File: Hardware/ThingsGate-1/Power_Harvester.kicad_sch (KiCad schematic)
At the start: 3 parts, among them U14 TL082, U5 BQ24650

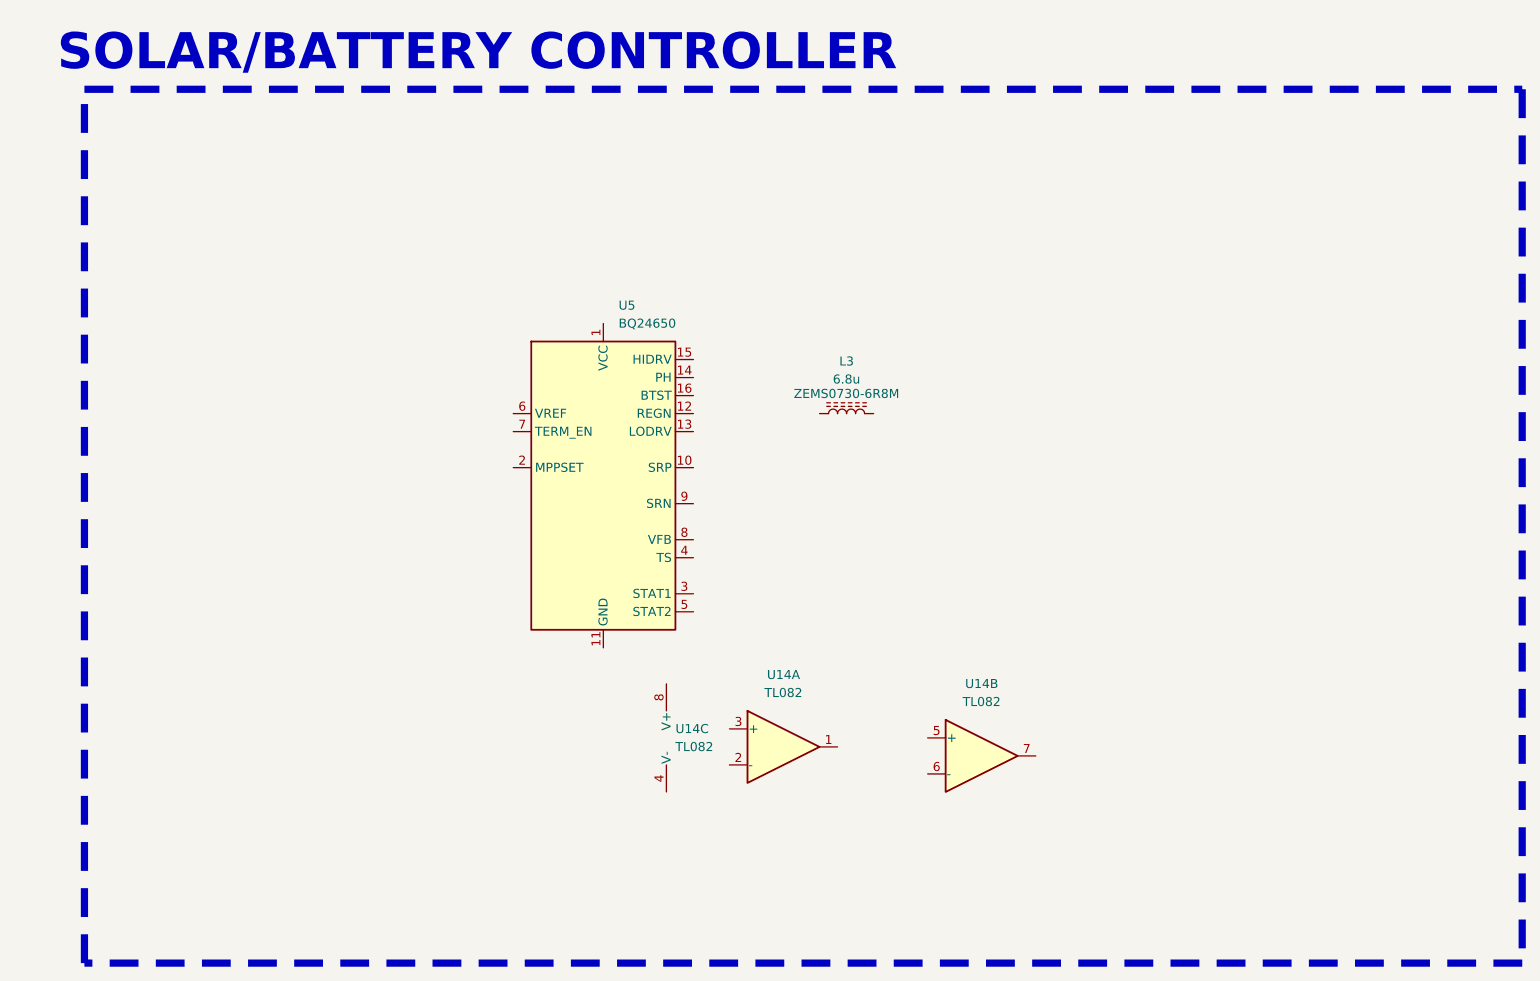
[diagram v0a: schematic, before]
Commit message: harvester schematic ready
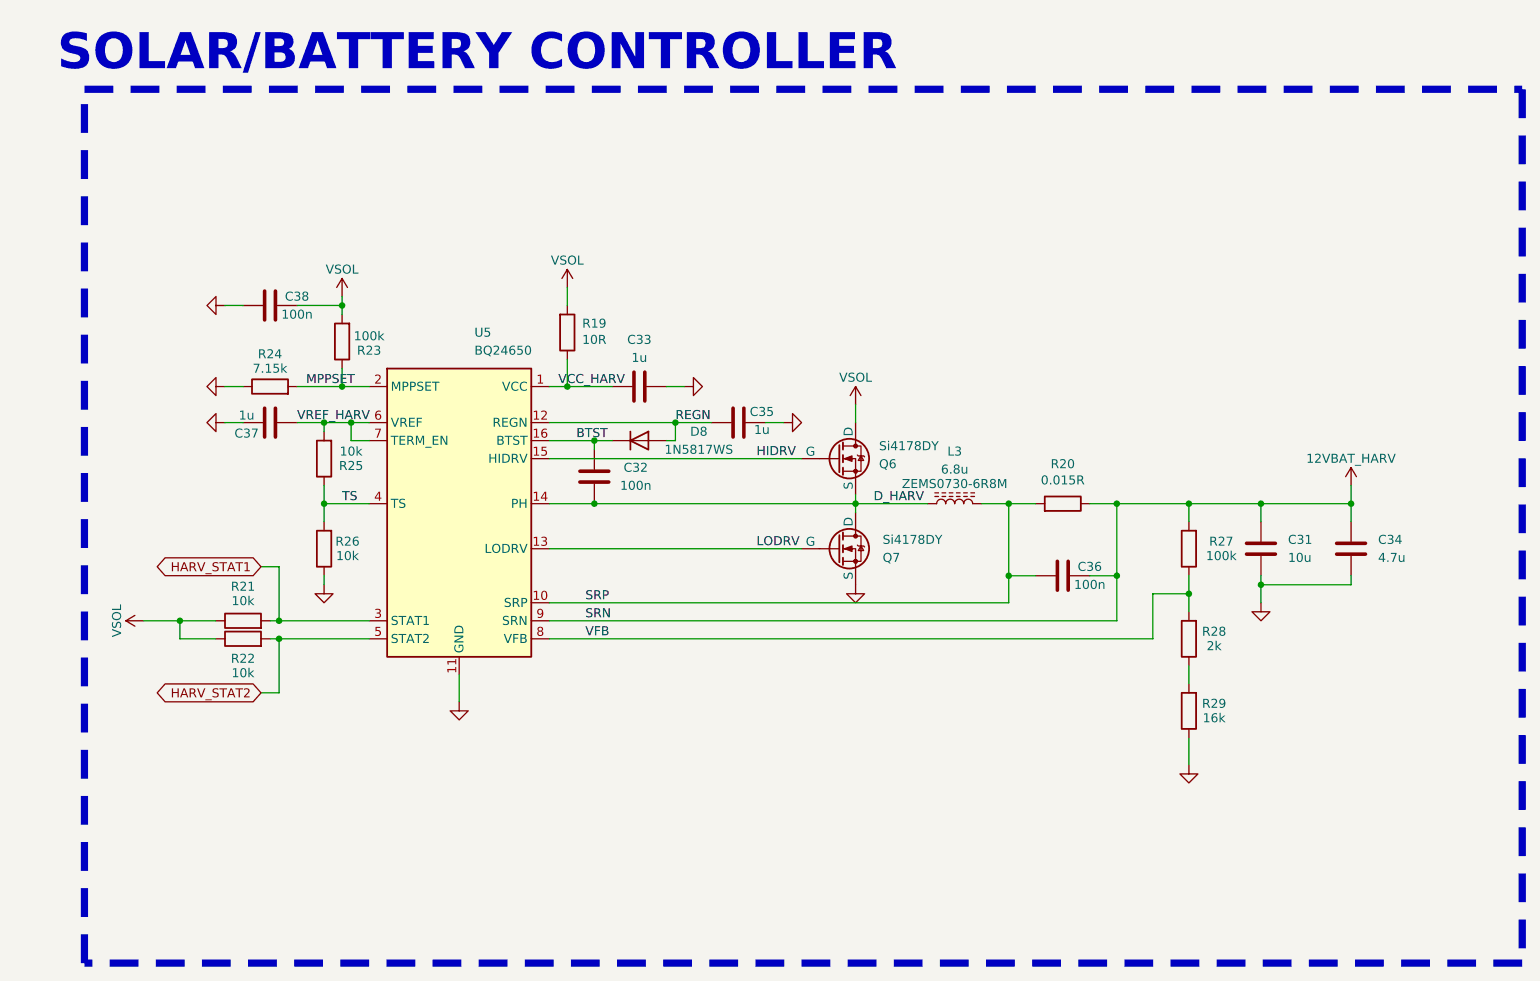
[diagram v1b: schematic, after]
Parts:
- removed U14: TL082, Package_SO:SOIC-8_3.9x4.9mm_P1.27mm, symbol Amplifier_Operational:TL082
- added C31: 10u, Fuse:Fuse_0805_2012Metric, symbol Device:C
- added C32, C36, C38: 100n, Capacitor_SMD:C_0603_1608Metric, symbol Device:C
- added C33, C35, C37: 1u, Fuse:Fuse_0805_2012Metric, symbol Device:C
- added C34: 4.7u, Fuse:Fuse_0805_2012Metric, symbol Device:C
- added D8: 1N5817WS, Diode_SMD:D_SOD-323, symbol Diode:1N4148WS
- added Q6, Q7: Si4178DY, ThingsGate-1:SO-8_3.9x4.9mm_P1.27mm, symbol ThingsGate-1:Si4178DY
- added R19: 10R, Resistor_SMD:R_1206_3216Metric, symbol Device:R
- added R20: 0.015R, Resistor_SMD:R_1206_3216Metric, symbol Device:R
- added R21, R22, R25, R26: 10k, Resistor_SMD:R_0603_1608Metric, symbol Device:R
- added R23, R27: 100k, Resistor_SMD:R_0603_1608Metric, symbol Device:R
- added R24: 7.15k, Resistor_SMD:R_0603_1608Metric, symbol Device:R
- added R28: 2k, Resistor_SMD:R_0603_1608Metric, symbol Device:R
- added R29: 16k, Resistor_SMD:R_0603_1608Metric, symbol Device:R
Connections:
- net D_HARV: now reaches L3.1
- net D_HARV: now also U5.14 (PH), C32.2, Q6.1 (S), Q6.2 (S), Q6.3 (S), Q7.5 (D), Q7.6 (D), Q7.7 (D), Q7.8 (D)
- net SRP: now reaches L3.2
- net SRP: now also U5.10 (SRP), C36.1, R20.2
- net VCC_HARV: now reaches U5.1 (VCC)
- net VCC_HARV: now also C33.1, R19.1
- net GND: now reaches U5.11 (GND), U5.17 (GND)
- net GND: now also C31.2, C33.2, C34.2, C35.2, C37.2, C38.1, Q7.1 (S), Q7.2 (S), Q7.3 (S), R24.1, R26.1, R29.1
- net REGN: now reaches U5.12 (REGN)
- net REGN: now also C35.1, D8.2 (A)
- net LODRV: now reaches U5.13 (LODRV)
- net LODRV: now also Q7.4 (G)
- net HIDRV: now reaches U5.15 (HIDRV)
- net HIDRV: now also Q6.4 (G)
- net BTST: now reaches U5.16 (BTST)
- net BTST: now also C32.1, D8.1 (K)
- net MPPSET: now reaches U5.2 (MPPSET)
- net MPPSET: now also R23.1, R24.2
- net HARV_STAT1: now reaches U5.3 (STAT1)
- net HARV_STAT1: now also R21.2
- net TS: now reaches U5.4 (TS)
- net TS: now also R25.1, R26.2
- net HARV_STAT2: now reaches U5.5 (STAT2)
- net HARV_STAT2: now also R22.2
- net VREF_HARV: now reaches U5.6 (VREF)
- net VREF_HARV: now also U5.7 (TERM_EN), C37.1, R25.2
- net VFB: now reaches U5.8 (VFB)
- net VFB: now also R27.1, R28.2
- net 12VBAT_HARV: now reaches U5.9 (SRN)
- net 12VBAT_HARV: now also C31.1, C34.1, C36.2, R20.1, R27.2
- new net: R28.1, R29.2
- new net VSOL: C38.2, Q6.5 (D), Q6.6 (D), Q6.7 (D), Q6.8 (D), R19.2, R21.1, R22.1, R23.2
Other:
- moved on the sheet: L3, U5
